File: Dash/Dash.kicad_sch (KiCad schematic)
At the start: 40 parts, among them CN1 NUCLEO-L432KC, J1 40 pin ZIF FPC Connector, J2 Nanofit Connector, U1 LF33_TO220, U2 LM7805_TO220, U3 BT817Q, U5 ISO1050DUB, U6 MCP2515-I/SO

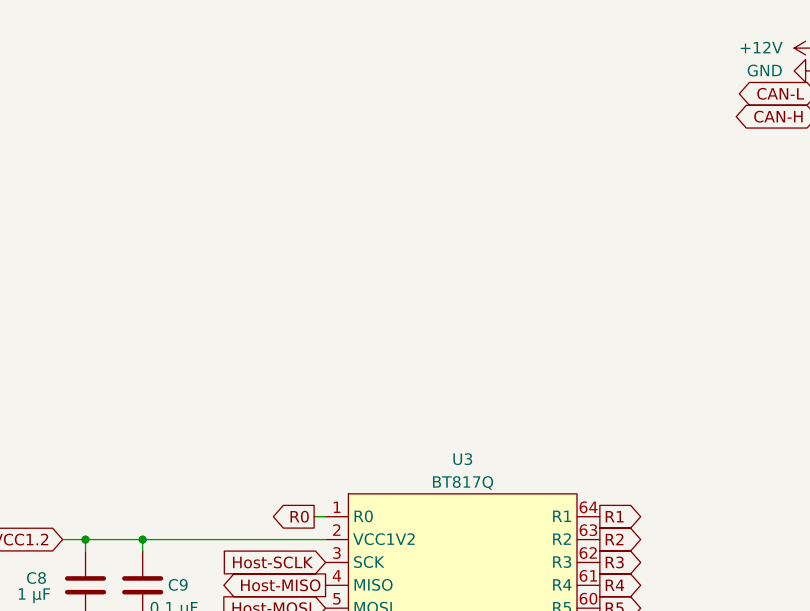
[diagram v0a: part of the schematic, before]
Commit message: Dash PCB revision 1
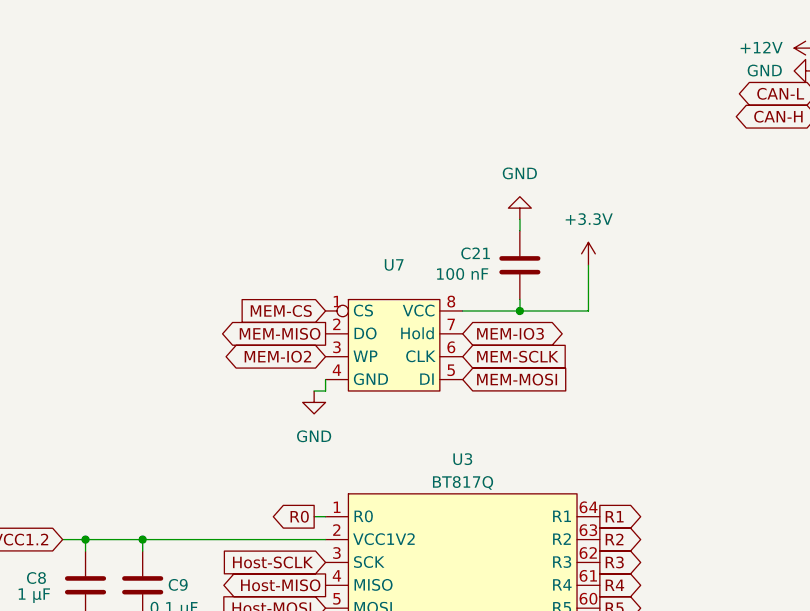
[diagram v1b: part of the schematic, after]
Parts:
- added C21: 100 nF, symbol Device:C
- added U7: ~, symbol FS_3_Global_Symbol_Library:W25Q40CLSNIG_TR
- D1: footprint Diode_SMD:D_0201_0603Metric -> FS_3_Global_Footprint_Library:US2H_TOS
- L1: footprint Inductor_SMD:L_1008_2520Metric -> Inductor_SMD:L_TDK_SLF7045
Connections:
- net +3.3V: now also C21.2, U7.8 (VCC)
- net GND: now also C21.1, U7.4 (GND)
- net MEM-CS: now also U7.1 (CS)
- net MEM-IO2: now also U7.3 (WP)
- net MEM-IO3: now also U7.7 (Hold)
- net MEM-MISO: now also U7.2 (DO)
- net MEM-MOSI: now also U7.5 (DI)
- net MEM-SCLK: now also U7.6 (CLK)

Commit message: fixed footprints for Dash
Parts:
- C21: footprint (none) -> Capacitor_SMD:C_0805_2012Metric
- U7: footprint (none) -> Package_SO:SOIC-8_3.9x4.9mm_P1.27mm
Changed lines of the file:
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@@
 			)
 		)
-		(property "Footprint" ""
+		(property "Footprint" "Capacitor_SMD:C_0805_2012Metric"
 			(at 230.8352 50.8 0)
 			(effects
@@
 			)
 		)
-		(property "Footprint" ""
+		(property "Footprint" "Package_SO:SOIC-8_3.9x4.9mm_P1.27mm"
 			(at 210.82 50.8 0)
 			(effects

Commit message: Fix footprint of flash chip
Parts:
- U7: footprint Package_SO:SOIC-8_3.9x4.9mm_P1.27mm -> Package_SO:SOIC-8_5.23x5.23mm_P1.27mm
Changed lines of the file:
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@@
 			)
 		)
-		(property "Footprint" "Package_SO:SOIC-8_3.9x4.9mm_P1.27mm"
+		(property "Footprint" "Package_SO:SOIC-8_5.23x5.23mm_P1.27mm"
 			(at 210.82 50.8 0)
 			(effects
